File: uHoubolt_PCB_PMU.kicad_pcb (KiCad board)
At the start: 2 copper layers, 117.8 x 90 mm, 11 parts, among them J1 Conn_01x02, J2 Conn_01x04, J3 Conn_01x03, SW1 Power_1, SW2 Power_2, SW3 Pyro_1, SW4 Pyro_2

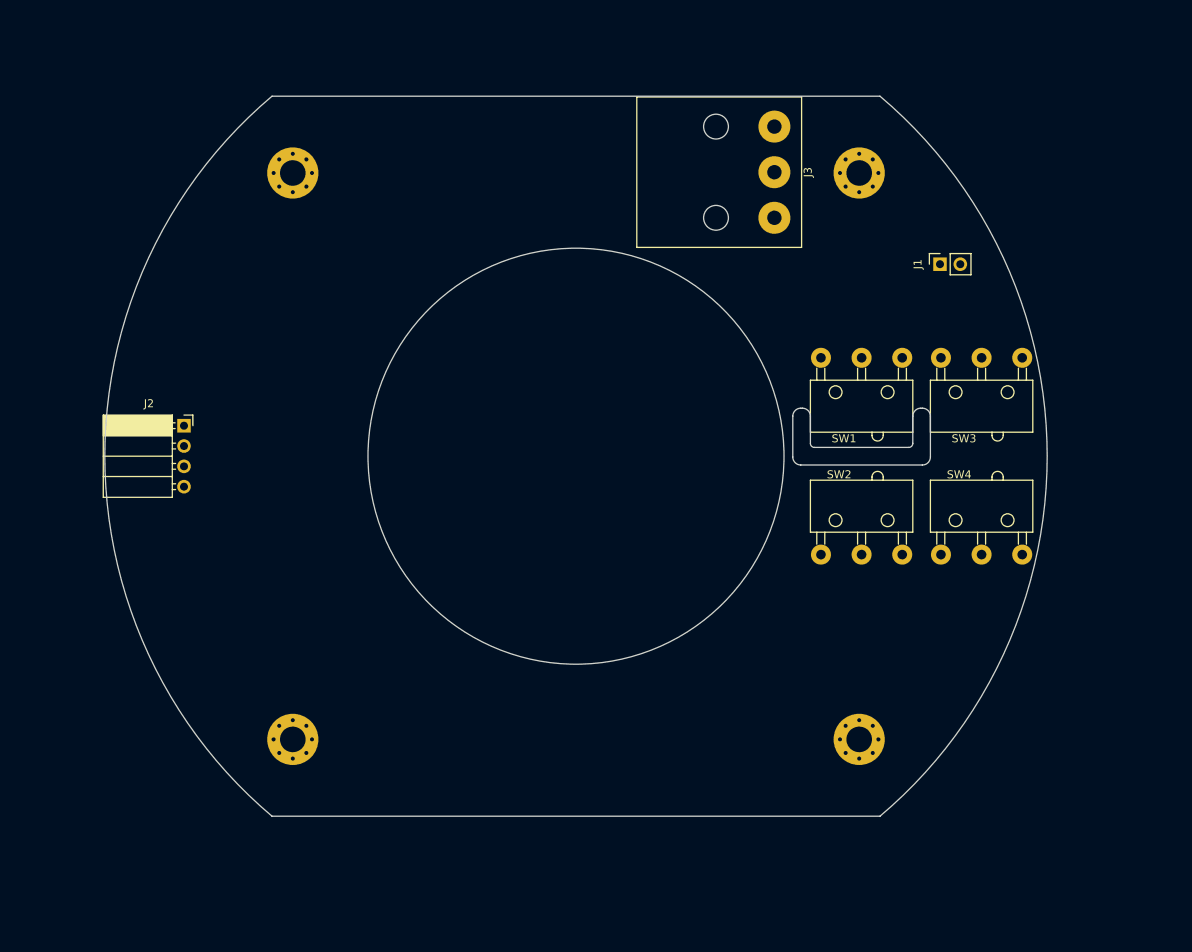
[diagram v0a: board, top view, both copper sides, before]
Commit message: PMU Layout
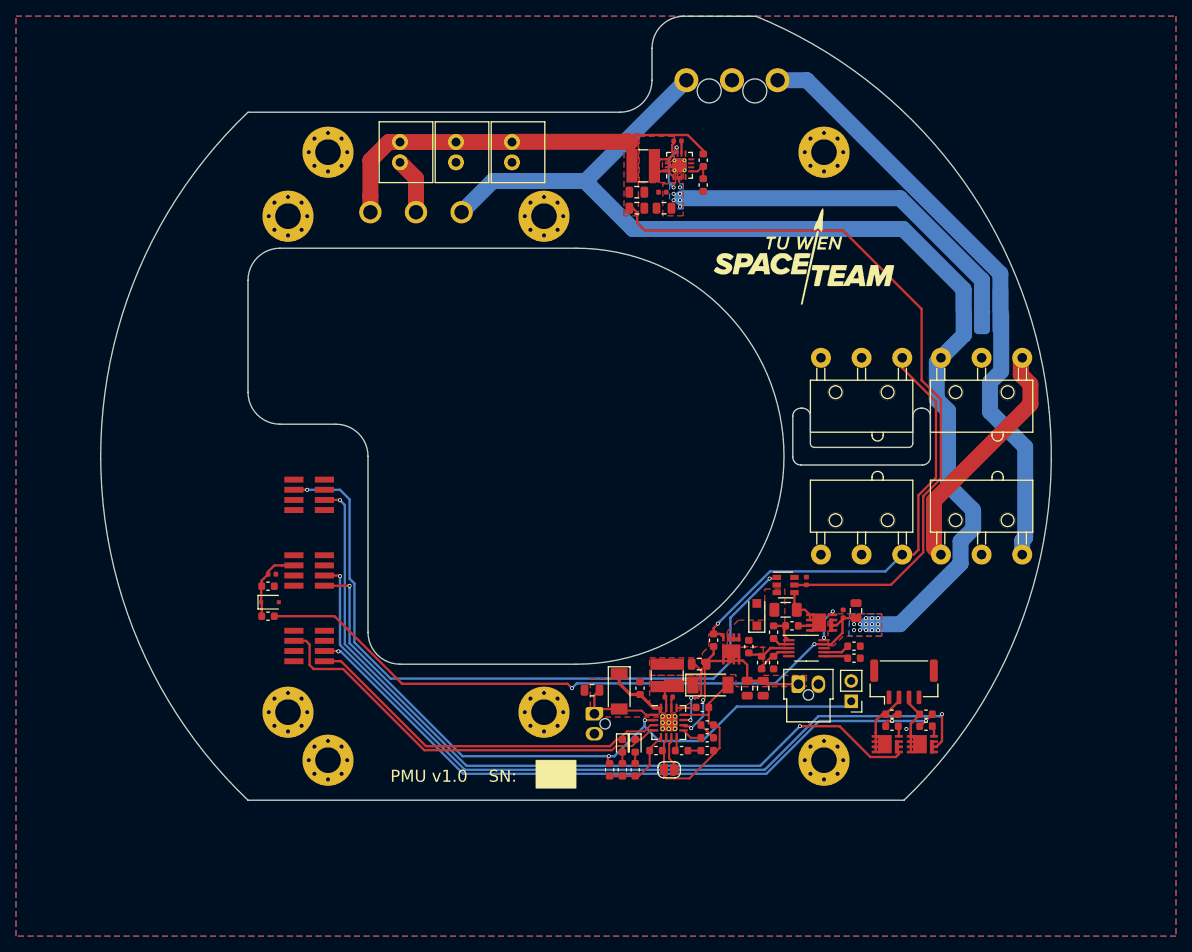
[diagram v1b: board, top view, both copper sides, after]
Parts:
- added C1: 470n, Capacitor_SMD:C_0603_1608Metric, F.Cu at (174.8, 125.2)
- added C10: 100n, Capacitor_SMD:C_0603_1608Metric, F.Cu at (155.8, 131.4)
- added C11: 100n, Capacitor_SMD:C_0402_1005Metric, F.Cu at (151.6, 130.1)
- added C12: 2.2n, Capacitor_SMD:C_0603_1608Metric, F.Cu at (156.4, 136.8)
- added C13: 2.2n, Capacitor_SMD:C_0603_1608Metric, F.Cu at (156.4, 133.6)
- added C14: 22u, Capacitor_SMD:C_0805_2012Metric, F.Cu at (161.4, 129.0)
- added C15: 22u, Capacitor_SMD:C_0805_2012Metric, F.Cu at (151.0, 69.0)
- added C16: 100n, Capacitor_SMD:C_0402_1005Metric, F.Cu at (150.8, 67.0)
- added C17: 22u, Capacitor_SMD:C_0805_2012Metric, F.Cu at (147.6, 69.0)
- added C18: 22u, Capacitor_SMD:C_0805_2012Metric, F.Cu at (163.4, 129.0)
- added C19: 100n, Capacitor_SMD:C_0402_1005Metric, F.Cu at (168.8, 115.6)
- added C2: 100n, Capacitor_SMD:C_0402_1005Metric, F.Cu at (102.0, 114.8)
- added C3: 100n, Capacitor_SMD:C_0402_1005Metric, F.Cu at (173.4, 119.7)
- added C4: 22u, Capacitor_SMD:C_0805_2012Metric, F.Cu at (175.0, 119.3)
- added C5: 100n, Capacitor_SMD:C_0402_1005Metric, F.Cu at (152.7, 60.6)
- added C6: 22u, Capacitor_SMD:C_0805_2012Metric, F.Cu at (147.6, 67.0)
- added C7: 22u, Capacitor_SMD:C_0805_2012Metric, F.Cu at (142.0, 129.2)
- added C8: 4.7u, Capacitor_SMD:C_0603_1608Metric, F.Cu at (150.0, 136.8)
- added C9: 4.7u, Capacitor_SMD:C_0603_1608Metric, F.Cu at (148.0, 129.0)
- added D1: 30V, Diode_SMD:D_SOD-123F, F.Cu at (162.6, 119.8)
- added D2: 3.3V, Diode_SMD:D_SOD-323F, F.Cu at (101.8, 118.2)
- added D3: LED, LED_SMD:LED_0603_1608Metric, F.Cu at (145.8, 136.2)
- added D4: LED, LED_SMD:LED_0603_1608Metric, F.Cu at (147.4, 136.2)
- added D5: PMEG3050EP, Diode_SMD:D_SOD-128, F.Cu at (145.4, 129.4)
- added D6: PMEG3050EP, Diode_SMD:D_SOD-128, F.Cu at (156.8, 128.6)
- added G1: SpaceTeam_LOGO, TXV_Library_Footprints:ST_Logo_new, F.Cu at (168.5, 75.0)
- added J4: Cam0, TXV_Library_Footprints:Molex_SL_1x2_Vertical, F.Cu at (118.0, 62.0)
- added J5: Batterycells, Connector_JST:JST_GH_BM04B-GHS-TBT_1x04-1MP_P1.25mm_Vertical, F.Cu at (181.0, 128.2)
- added J6: Cam1, TXV_Library_Footprints:Molex_SL_1x2_Vertical, F.Cu at (125.0, 62.0)
- added J7: Cam2, TXV_Library_Footprints:Molex_SL_1x2_Vertical, F.Cu at (132.0, 62.0)
- added JP1: Jumper_3_Open, TXV_Library_Footprints:Jumper3_6x2mm, B.Cu at (190.8, 81.8)
- added JP2: Jumper_2_Open, Jumper:SolderJumper-2_P1.3mm_Open_RoundedPad1.0x1.5mm, F.Cu at (151.7, 139.2)
- added L1: 4.7u, TXV_Library_Footprints:SRN4018TA-4R7M, F.Cu at (148.4, 63.7)
- added L2: 4.7u, TXV_Library_Footprints:SRN4018TA-4R7M, F.Cu at (151.4, 127.4)
- added Q1: Q_PMOS_DGS, TXV_Library_Footprints:PG_TSDSON-8, F.Cu at (159.4, 124.0)
- added Q2: BSZ0902NSATMA1, TXV_Library_Footprints:PG_TSDSON-8, F.Cu at (170.8, 120.8)
- added Q3: Q_PMOS_DGS, TXV_Library_Footprints:PG_TSDSON-8, F.Cu at (183.4, 136.0)
- added Q4: Q_PMOS_DGS, TXV_Library_Footprints:PG_TSDSON-8, F.Cu at (179.0, 136.0)
- added R1: 10k, Resistor_SMD:R_0603_1608Metric, F.Cu at (157.2, 123.0)
- added R10: R, Resistor_SMD:R_0603_1608Metric, F.Cu at (101.5, 120.0)
- added R11: R, Resistor_SMD:R_0603_1608Metric, F.Cu at (101.5, 116.2)
- added R14: 200, Resistor_SMD:R_0603_1608Metric, F.Cu at (183.8, 133.8)
- added R15: 10k, Resistor_SMD:R_0603_1608Metric, F.Cu at (183.8, 132.2)
- added R18: 200, Resistor_SMD:R_0603_1608Metric, F.Cu at (179.5, 133.8)
- added R19: 10k, Resistor_SMD:R_0603_1608Metric, F.Cu at (179.5, 132.2)
- added R2: R, Resistor_SMD:R_0603_1608Metric, F.Cu at (161.6, 123.8)
- added R20: R, Resistor_SMD:R_0603_1608Metric, F.Cu at (155.9, 63.0)
- added R21: R, Resistor_SMD:R_0603_1608Metric, F.Cu at (155.9, 66.1)
- added R22: 10k, Resistor_SMD:R_0603_1608Metric, F.Cu at (144.2, 139.2)
- added R23: 120, Resistor_SMD:R_0603_1608Metric, F.Cu at (145.8, 139.2)
- added R24: 120, Resistor_SMD:R_0603_1608Metric, F.Cu at (147.4, 139.2)
- added R25: 750, Resistor_SMD:R_0603_1608Metric, F.Cu at (156.4, 135.2)
- added R26: 2.5k, Resistor_SMD:R_0603_1608Metric, F.Cu at (153.2, 136.8)
- added R27: 140m, Resistor_SMD:R_0805_2012Metric, F.Cu at (155.4, 126.0)
- added R3: R, Resistor_SMD:R_0603_1608Metric, F.Cu at (163.2, 125.8)
- added R4: R, Resistor_SMD:R_0603_1608Metric, F.Cu at (164.7, 125.8)
- added R5: NP, Resistor_SMD:R_0603_1608Metric, F.Cu at (164.7, 122.0)
- added R6: 2m, Resistor_SMD:R_1206_3216Metric, F.Cu at (166.2, 119.2)
- added R7: 0R, Resistor_SMD:R_0603_1608Metric, F.Cu at (167.0, 121.2)
- added R9: 47k, Resistor_SMD:R_0603_1608Metric, F.Cu at (174.8, 123.8)
- added TH1: Thermistor_NTC, Connector_PinHeader_2.54mm:PinHeader_1x02_P2.54mm_Vertical, F.Cu at (174.4, 130.6)
- added U1: LM5069, Package_SO:VSSOP-10_3x3mm_P0.5mm, F.Cu at (168.8, 124.0)
- added U2: LMP8640 F, Package_TO_SOT_SMD:SOT-23-6, F.Cu at (166.2, 116.1)
- added U3: TS30041, Package_DFN_QFN:QFN-16-1EP_3x3mm_P0.5mm_EP1.75x1.75mm_ThermalVias, F.Cu at (152.9, 63.6)
- added U4: MP26123, Package_DFN_QFN:QFN-16-1EP_4x4mm_P0.65mm_EP2.15x2.15mm_ThermalVias, F.Cu at (151.6, 133.3)
- added U5: ECU, TXV_Library_Footprints:ECU_Footprint_simple, F.Cu at (120.0, 101.0)
- H1, H2, H3, H4: value MountingHole_Pad -> M3
- J1: value Conn_01x02 -> Umbilical; footprint Connector_PinSocket_2.54mm:PinSocket_1x02_P2.54mm_Vertical -> TXV_Library_Footprints:Molex_Nano-Fit_105309-xx02_1x02_P2.50mm_Vertical; moved to B.Cu
- J2: value Conn_01x04 -> Battery; footprint Connector_PinSocket_2.54mm:PinSocket_1x04_P2.54mm_Horizontal -> TXV_Library_Footprints:Molex_Nano-Fit_105309-xx02_1x02_P2.50mm_Vertical
- J3: value Conn_01x03 -> Power; footprint TXV_Library_Footprints:Molex_MegaFit_1x03 -> TXV_Library_Footprints:Molex_MegaFit_1x03_Vertical; moved to B.Cu
- moved J2 83.3 mm to (167.8, 128.5), turned to 90 degrees
- moved J1 70.9 mm to (142.3, 132.2), turned to 180 degrees
- moved J3 11.7 mm to (159.5, 53.0), turned to 180 degrees
- moved H1 5.11 mm to (109.0, 62.0)
- moved H2 5.11 mm to (171.0, 62.0)
- moved H3 5.11 mm to (109.0, 138.0)
- moved H4 5.11 mm to (171.0, 138.0)
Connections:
- H1 pad 1: Net-(H1-Pad1) -> GND
- H2 pad 1: Net-(H2-Pad1) -> GND
- H3 pad 1: Net-(H3-Pad1) -> GND
- H4 pad 1: Net-(H4-Pad1) -> GND
- J1 pad 1: Net-(J1-Pad1) -> /Vcharge
- J1 pad 2: Net-(J1-Pad2) -> GND
- J2 pad 1: Net-(J2-Pad1) -> /Vbat
- J2 pad 2: Net-(J2-Pad2) -> GND
- J3 pad 1: Net-(J3-Pad1) -> +12V
- J3 pad 2: Net-(J3-Pad2) -> GND
- J3 pad 3: Net-(J3-Pad3) -> PYRO
- SW1 pad 1: Net-(SW1-Pad1) -> GND
- SW1 pad 2: Net-(SW1-Pad2) -> Net-(Q1-Pad2)
- SW1 pad 3: Net-(SW1-Pad3) -> (no net)
- SW2 pad 1: Net-(SW2-Pad1) -> GND
- SW2 pad 2: Net-(SW2-Pad2) -> Net-(Q1-Pad2)
- SW2 pad 3: Net-(SW2-Pad3) -> (no net)
- SW3 pad 1: Net-(SW3-Pad1) -> +12V
- SW3 pad 3: Net-(SW3-Pad3) -> GND
- SW4 pad 1: Net-(SW4-Pad1) -> Net-(SW3-Pad2)
- SW4 pad 2: Net-(SW4-Pad2) -> PYRO
- SW4 pad 3: Net-(SW4-Pad3) -> GND
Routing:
- net +12V: track 0.00 -> 225.1 mm, vias 0 -> 15
- net +5V: track 0.00 -> 146.2 mm
- net Net-(Q3-Pad1): track 0.00 -> 100.1 mm, vias 0 -> 2
- net Net-(Q4-Pad1): track 0.00 -> 99.8 mm, vias 0 -> 2
- net Net-(R14-Pad2): track 0.00 -> 89.4 mm, vias 0 -> 3
- net /SUPPLY_CURRENT_SENSE: track 0.00 -> 88.7 mm, vias 0 -> 2
- net /NTC: track 0.00 -> 86.7 mm, vias 0 -> 3
- net PYRO: track 0.00 -> 75.0 mm
- net Net-(Q1-Pad2): track 0.00 -> 58.5 mm, vias 0 -> 1
- net /~CHGOK: track 0.00 -> 53.5 mm
- net Net-(C15-Pad2): track 0.00 -> 53.4 mm, vias 0 -> 8
- net /~ACOK: track 0.00 -> 47.0 mm
- net GND: track 0.00 -> 37.6 mm, vias 0 -> 1
- net Net-(SW3-Pad2): track 0.00 -> 30.5 mm
- net /Vbat: track 0.00 -> 27.6 mm, vias 0 -> 2
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- added copper zone on B.Cu, net +12V
- added copper zone on F.Cu, net +12V
- added copper zone on F.Cu, net +5V
- added copper zone on F.Cu, net /Vbat
- added copper zone on F.Cu, net /Vcharge
- added copper zone on F.Cu, net /Vin
- added copper zone on B.Cu, net GND
- added copper zone on F.Cu, net GND
- added copper zone on F.Cu, net Net-(C11-Pad1)
- added copper zone on B.Cu, net Net-(C15-Pad2)
- added copper zone on F.Cu, net Net-(C15-Pad2)
- added copper zone on F.Cu, net Net-(C5-Pad1)
- added copper zone on F.Cu, net Net-(L2-Pad2)
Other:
- board size 117.8 x 90 mm -> 118.8 x 98 mm
- rule via_min_size: 0.4 -> 0.3
- board text added: "PMU v1.0 SN:"
- board text removed: "Leinenseite"
- board text removed: "Schaltbare Ausgänge"

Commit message: New Layout
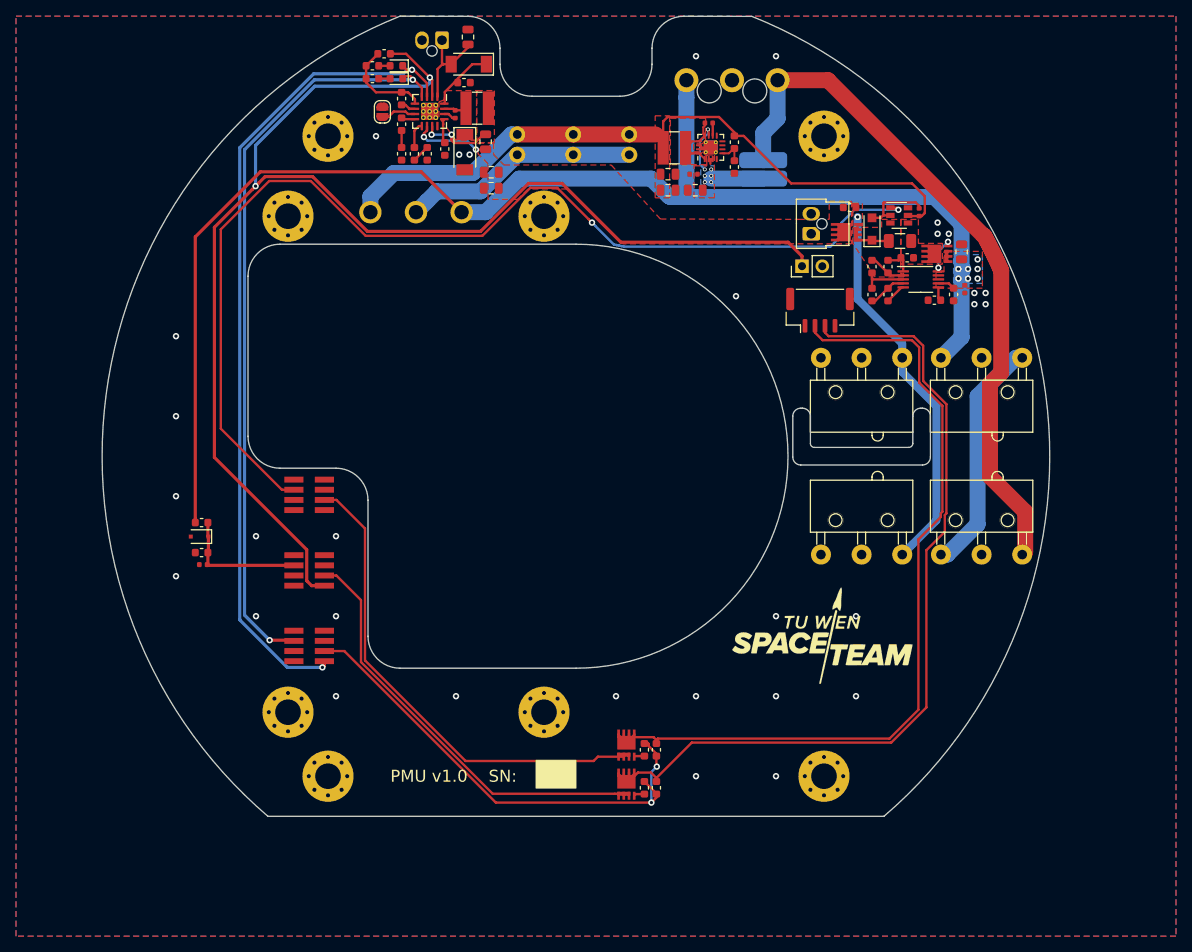
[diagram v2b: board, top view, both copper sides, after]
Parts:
- J4, J6, J7: moved to B.Cu
- moved R22 93.8 mm to (116.0, 49.7), turned to 0 degrees
- moved R23 93.4 mm to (114.5, 51.2), turned to 0 degrees
- moved R24 92.4 mm to (114.5, 52.8), turned to 0 degrees
- moved JP2 89.7 mm to (115.8, 57.0), turned to 90 degrees
- moved D3 89.6 mm to (117.5, 51.2), turned to 180 degrees
- moved D4 88.6 mm to (117.5, 52.8), turned to 180 degrees
- moved C8 87.5 mm to (118.2, 55.3), turned to 270 degrees
- moved J1 86.3 mm to (123.2, 48.0), turned to 90 degrees
- moved R26 85.8 mm to (118.2, 58.5), turned to 90 degrees
- moved C12 83.8 mm to (118.2, 62.2), turned to 270 degrees
- moved C7 83.1 mm to (126.5, 47.6), turned to 90 degrees
- moved U4 82.0 mm to (121.7, 56.9), turned to 270 degrees
- moved R25 81.7 mm to (119.8, 62.2), turned to 90 degrees
- moved D5 80.6 mm to (126.6, 51.0), turned to 180 degrees
- moved C13 79.5 mm to (121.4, 62.2), turned to 270 degrees
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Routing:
- net /Cell1: track 9.40 -> 109.3 mm
- net /Cell2: track 9.85 -> 107.0 mm
- net /NTC: track 86.7 -> 177.3 mm, vias 3 -> 2
- net +5V: track 146.2 -> 85.8 mm
- net /~ACOK: track 47.0 -> 103.9 mm, vias 0 -> 2
- net +12V: track 225.1 -> 174.0 mm, vias 15 -> 7
- net /SUPPLY_CURRENT_SENSE: track 88.7 -> 136.7 mm
- net Net-(Q3-Pad1): track 100.1 -> 53.3 mm, vias 2 -> 0
- net /~CHGOK: track 53.5 -> 94.7 mm, vias 0 -> 2
- net Net-(C15-Pad2): track 53.4 -> 14.2 mm, vias 8 -> 7
- net Net-(Q4-Pad1): track 99.8 -> 60.8 mm, vias 2 -> 0
- net Net-(R14-Pad2): track 89.4 -> 60.8 mm, vias 3 -> 2
- net /Vbat: track 27.6 -> 9.90 mm
- net PYRO: track 75.0 -> 87.5 mm
- net Net-(Q2-Pad3): track 10.7 -> 0.00 mm
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- added copper zone on F.Cu, net Net-(Q1-Pad2)
- added copper zone on F.Cu, net Net-(Q2-Pad3)
- removed copper zone on F.Cu, net /Vcharge
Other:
- board size 118.8 x 98 mm -> 118.5 x 100 mm
- board text removed: "Akkumanagement"
